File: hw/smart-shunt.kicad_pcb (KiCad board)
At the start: 2 copper layers, 80.3 x 50.3 mm, 36 parts, among them J1 V supply, J2 V bus <80, J3 V bus >80, J4 Conn_01x01_Female, J5 Conn_01x01_Female, J6 GND, U1 XL7005A, U2 INA228, U3 ESP-12F

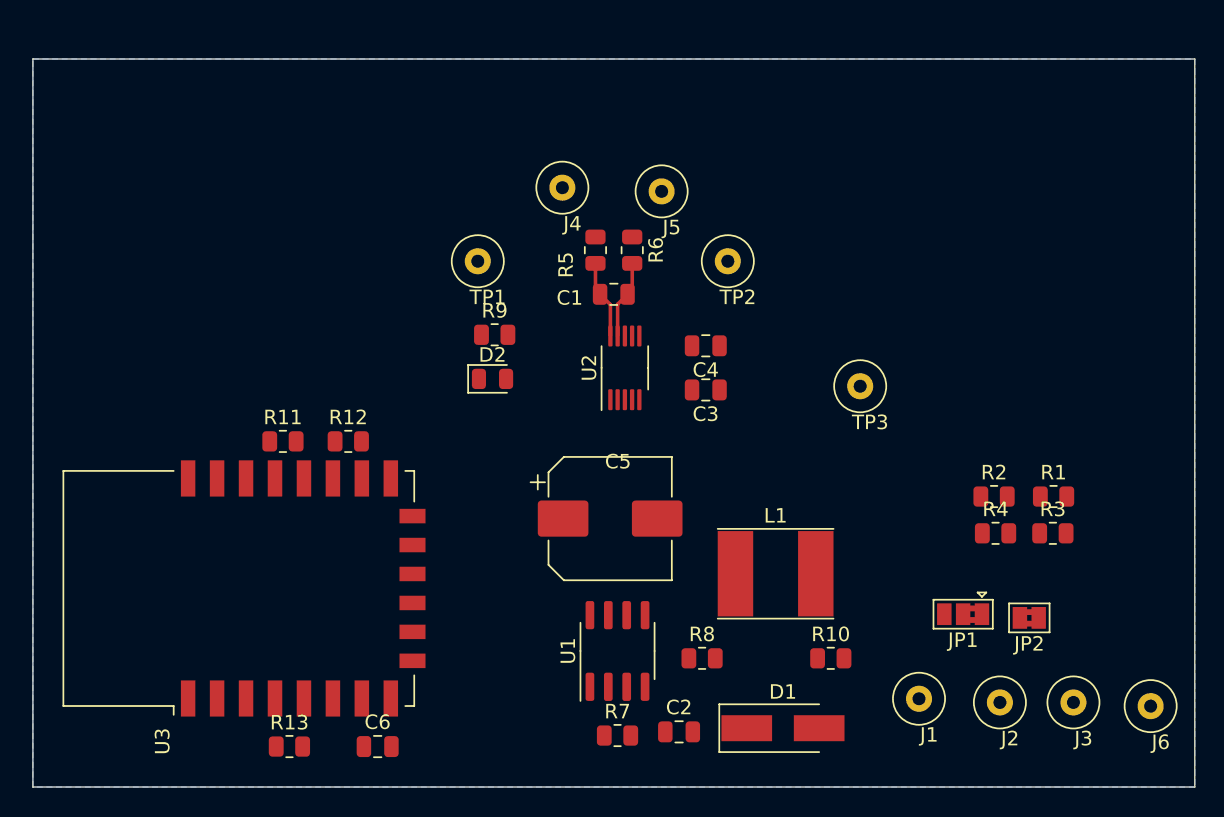
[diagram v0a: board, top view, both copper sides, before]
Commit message: finished pcb
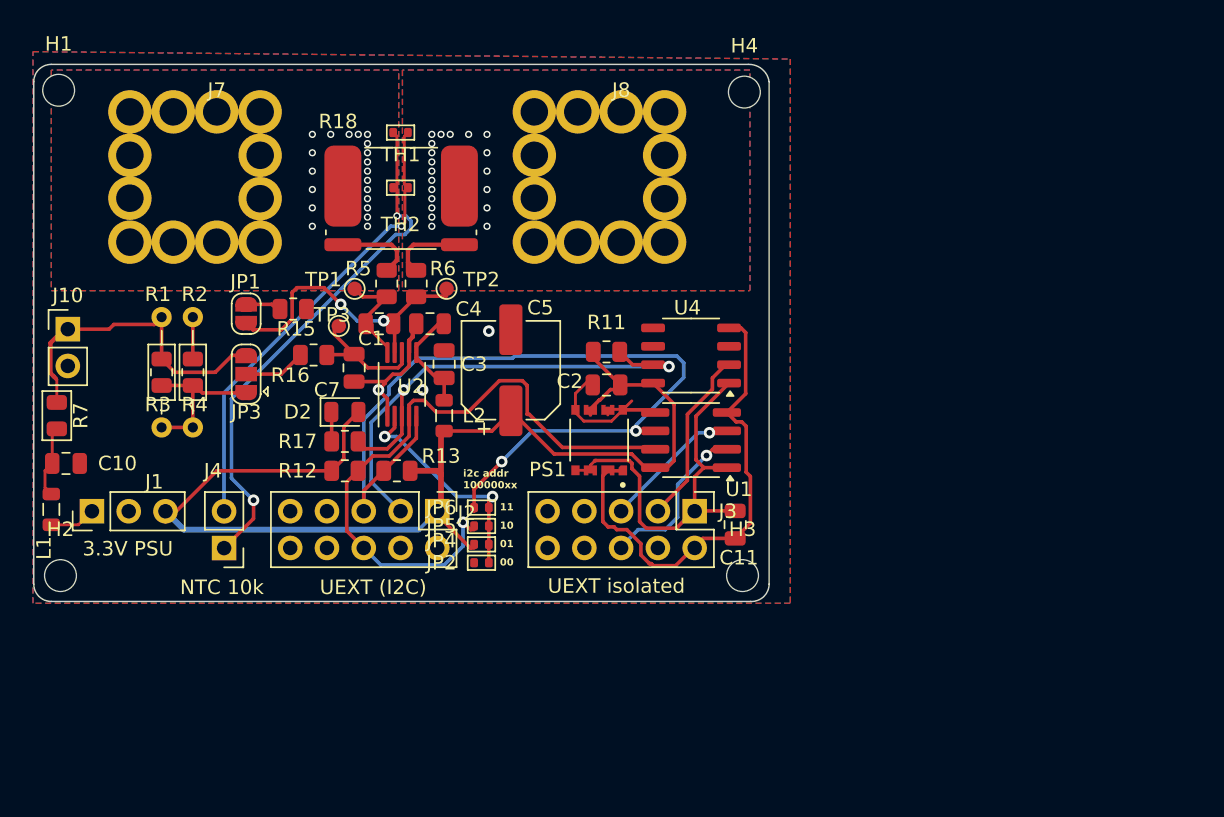
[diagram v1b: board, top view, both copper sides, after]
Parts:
- removed C6: 0.1uF, Capacitor_SMD:C_0805_2012Metric
- removed D1: SS310, Diode_SMD:D_SMA_Handsoldering
- removed J5: Conn_01x01_Female, TestPoint:TestPoint_Loop_D3.50mm_Drill0.9mm_Beaded
- removed J6: GND, TestPoint:TestPoint_Loop_D3.50mm_Drill0.9mm_Beaded
- removed R10: 33k, Resistor_SMD:R_0805_2012Metric
- removed R8, R9: 10k, Resistor_SMD:R_0805_2012Metric
- removed U3: ESP-12F, RF_Module:ESP-12E
- added C10: 1uF 100V, Capacitor_SMD:C_0805_2012Metric, F.Cu at (81.0, 99.6)
- added C11: 100nF, Capacitor_SMD:C_0805_2012Metric, F.Cu at (127.3, 103.8)
- added C7: 0.1uF, Capacitor_SMD:C_0805_2012Metric, F.Cu at (100.9, 93.0)
- added H1: MountingHole, MountingHole:MountingHole_2.2mm_M2, F.Cu at (80.5, 73.8)
- added H2: MountingHole, MountingHole:MountingHole_2.2mm_M2, F.Cu at (80.6, 107.3)
- added H3: MountingHole, MountingHole:MountingHole_2.2mm_M2, F.Cu at (127.8, 107.3)
- added H4: MountingHole, MountingHole:MountingHole_2.2mm_M2, F.Cu at (127.9, 73.9)
- added J10: Conn_01x02_Pin, Connector_PinHeader_2.54mm:PinHeader_1x02_P2.54mm_Vertical, F.Cu at (81.2, 90.3)
- added J7: Screw_Terminal_01x01, open-pe:Wuerth_PowerPlus_M5_Nut, F.Cu at (91.4, 81.3)
- added J8: Screw_Terminal_01x01, open-pe:Wuerth_PowerPlus_M5_Nut, F.Cu at (119.4, 81.3)
- added JP3: Jumper_3_Open, Jumper:SolderJumper-3_P1.3mm_Open_RoundedPad1.0x1.5mm, F.Cu at (93.5, 93.4)
- added JP4: SolderJumper_2_Open, PCM_Resistor_SMD_AKL:R_0402_1005Metric, F.Cu at (109.7, 105.2)
- added JP5: SolderJumper_2_Open, PCM_Resistor_SMD_AKL:R_0402_1005Metric, F.Cu at (109.7, 103.9)
- added JP6: SolderJumper_2_Open, PCM_Resistor_SMD_AKL:R_0402_1005Metric, F.Cu at (109.7, 102.6)
- added L2: LBR2012T101K, Inductor_SMD:L_0805_2012Metric, F.Cu at (107.1, 96.3)
- added PS1: MIE1W0505BGLVH-3R-Z, open-pe:CONV_MIE1W0505BGLVH-3R-Z, F.Cu at (117.9, 98.0)
- added R15: 10, Resistor_SMD:R_0805_2012Metric, F.Cu at (96.7, 88.9)
- added R16: 100, Resistor_SMD:R_0805_2012Metric, F.Cu at (98.1, 92.1)
- added R17: 10k, Resistor_SMD:R_0805_2012Metric, F.Cu at (100.3, 98.0)
- added R18: R_Shunt, Resistor_SMD:R_Shunt_Isabellenhuette_BVR4026, F.Cu at (104.2, 81.3)
- added TH1: Thermistor_NTC, PCM_Resistor_SMD_AKL:R_0402_1005Metric, F.Cu at (104.1, 76.7)
- added TH2: Thermistor_NTC, PCM_Resistor_SMD_AKL:R_0402_1005Metric, F.Cu at (104.1, 80.5)
- added U4: TPT7721-SO1R, Package_SO:SOP-8_3.9x4.9mm_P1.27mm, F.Cu at (124.2, 92.1)
- C2: value 33nF -> 100nF
- C5: value 100uF -> 22uF; footprint Capacitor_SMD:CP_Elec_8x10 -> Capacitor_SMD:CP_Elec_6.3x5.9
- J1: value V supply -> Conn_01x03_Socket; footprint TestPoint:TestPoint_Loop_D3.50mm_Drill0.9mm_Beaded -> Connector_PinHeader_2.54mm:PinHeader_1x03_P2.54mm_Vertical
- J2: value V bus <80 -> UEXT_Slave; footprint TestPoint:TestPoint_Loop_D3.50mm_Drill0.9mm_Beaded -> Connector_PinHeader_2.54mm:PinHeader_2x05_P2.54mm_Vertical
- J3: value V bus >80 -> UEXT_Slave2; footprint TestPoint:TestPoint_Loop_D3.50mm_Drill0.9mm_Beaded -> Connector_PinHeader_2.54mm:PinHeader_2x05_P2.54mm_Vertical
- J4: value Conn_01x01_Female -> Conn_01x02_Pin; footprint TestPoint:TestPoint_Loop_D3.50mm_Drill0.9mm_Beaded -> Connector_PinHeader_2.54mm:PinHeader_1x02_P2.54mm_Vertical
- JP1: value Jumper_3_Bridged12 -> Jumper_2_Open; footprint Jumper:SolderJumper-3_P1.3mm_Bridged2Bar12_Pad1.0x1.5mm -> Jumper:SolderJumper-2_P1.3mm_Open_RoundedPad1.0x1.5mm
- JP2: value Jumper_2_Open -> SolderJumper_2_Open; footprint Jumper:SolderJumper-2_P1.3mm_Bridged2Bar_Pad1.0x1.5mm -> PCM_Resistor_SMD_AKL:R_0402_1005Metric
- L1: value 100uH -> 22uH; footprint Inductor_SMD:L_Taiyo-Yuden_NR-60xx_HandSoldering -> Inductor_SMD:L_0805_2012Metric
- R1, R2: footprint Resistor_SMD:R_0805_2012Metric -> Resistor_THT:R_Axial_DIN0204_L3.6mm_D1.6mm_P7.62mm_Horizontal
- R7: value 33k -> 10; footprint Resistor_SMD:R_0805_2012Metric -> PCM_Resistor_SMD_AKL:R_0805_2012Metric
- TP1, TP2, TP3: footprint TestPoint:TestPoint_Loop_D3.50mm_Drill0.9mm_Beaded -> TestPoint:TestPoint_Pad_D1.0mm
- U1: value XL7005A -> TPT72616-SO1R
- moved R3 62.6 mm to (87.6, 93.3), turned to 90 degrees
- moved R1 61.8 mm to (87.6, 97.1), turned to 90 degrees
- moved J1 58.6 mm to (82.8, 102.9), turned to 90 degrees
- moved R2 56.7 mm to (89.8, 89.5), turned to -90 degrees
- moved R4 56.6 mm to (89.8, 93.3), turned to -90 degrees
- moved JP1 53.7 mm to (93.5, 89.2), turned to -90 degrees
- moved L1 50.2 mm to (80.0, 102.7), turned to 90 degrees
- moved R7 44.6 mm to (80.4, 96.3), turned to 90 degrees
- moved J2 41.1 mm to (106.7, 102.9), turned to -90 degrees
- moved JP2 38.0 mm to (109.7, 106.4)
- moved TP3 36.3 mm to (99.9, 90.1)
- moved J4 34.1 mm to (91.9, 105.4), turned to 180 degrees
- moved J3 29.3 mm to (124.5, 102.9), turned to -90 degrees
- moved C2 24.5 mm to (118.4, 94.1), turned to 180 degrees
- moved R11 23.2 mm to (118.4, 91.9), turned to 180 degrees
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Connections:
- C1 pad 2: Net-(TP2-Pad1) -> Net-(JP1-B)
- C2 pad 2: Net-(C2-Pad2) -> GND
- C3 pad 1: +3.3V -> Net-(U2-VS)
- C4 pad 1: +3.3V -> Net-(U2-VS)
- C5 pad 2: Net-(C5-Pad2) -> GND
- D2 pad 2: Alert -> +3.3V
- J1 pad 1: Net-(U1-Pad1) -> Net-(J1-Pin_1)
- J2 pad 1: Vbus -> +3.3V
- J3 pad 1: Net-(J3-Pad1) -> +3.3V2
- J4 pad 1: Net-(J4-Pad1) -> Net-(J4-Pin_1)
- JP1 pad 1: Vbus -> Net-(JP1-A)
- JP1 pad 2: Net-(JP1-Pad2) -> Net-(JP1-B)
- JP2 pad 1: Net-(JP2-Pad1) -> A0
- JP2 pad 2: Vbus -> GND
- L1 pad 1: Net-(D1-Pad1) -> Net-(J1-Pin_1)
- L1 pad 2: +3.3V -> Net-(C10-Pad2)
- R1 pad 1: Net-(JP2-Pad1) -> Net-(JP3-A)
- R1 pad 2: Net-(J3-Pad1) -> Vin
- R2 pad 2: Net-(JP2-Pad1) -> Net-(JP3-A)
- R3 pad 1: Net-(JP2-Pad1) -> Net-(JP3-A)
- R3 pad 2: Net-(J3-Pad1) -> Vin
- R4 pad 2: Net-(JP2-Pad1) -> Net-(JP3-A)
- R5 pad 1: Net-(J4-Pad1) -> Shunt+
- R6 pad 1: Net-(J5-Pad1) -> Shunt-
- R6 pad 2: Net-(TP2-Pad1) -> Net-(JP1-B)
- R7 pad 1: +3.3V -> Net-(C10-Pad2)
- R7 pad 2: Net-(C2-Pad2) -> Vin
- TP2 pad 1: Net-(TP2-Pad1) -> Net-(JP1-B)
- TP3 pad 1: Vbus -> Net-(U2-Vbus)
- U1 pad 1: Net-(U1-Pad1) -> +3.3V2
- U1 pad 2: Net-(D1-Pad1) -> SDA2
- U1 pad 3: Net-(C2-Pad2) -> SCL2
- U1 pad 4: Net-(C5-Pad2) -> GND2
- U1 pad 5: Net-(C5-Pad2) -> GND
- U1 pad 6: Net-(C5-Pad2) -> SCL
- U1 pad 7: Net-(C5-Pad2) -> SDA
- U1 pad 8: Net-(C5-Pad2) -> +3.3V
- U2 pad 2: GND -> A0
- U2 pad 6: +3.3V -> Net-(U2-VS)
- U2 pad 8: Vbus -> Net-(U2-Vbus)
- U2 pad 9: Net-(TP2-Pad1) -> Net-(JP1-B)
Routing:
- net +3.3V: track 0.00 -> 81.9 mm
- net SCL: track 0.00 -> 60.2 mm, vias 0 -> 2
- net SDA: track 0.00 -> 44.8 mm, vias 0 -> 1
- net Alert: track 0.00 -> 39.3 mm, vias 0 -> 2
- net Net-(J4-Pin_1): track 0.00 -> 36.6 mm, vias 0 -> 2
- net GND2: track 0.00 -> 33.9 mm
- net Net-(J4-Pin_2): track 0.00 -> 32.2 mm, vias 0 -> 1
- net +3.3V2: track 0.00 -> 28.2 mm
- net GND: track 0.00 -> 23.2 mm, vias 0 -> 3
- net Vin: track 0.00 -> 21.7 mm
- net Net-(JP1-B): track 0.00 -> 20.7 mm, vias 0 -> 2
- net A0: track 0.00 -> 14.9 mm, vias 0 -> 2
- net Alert2: track 0.00 -> 12.2 mm
- net SDA2: track 0.00 -> 11.4 mm, vias 0 -> 1
- net Net-(JP3-A): track 0.00 -> 10.6 mm
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- added copper zone on F.Cu, net GND
- added copper zone on B.Cu, net P+
- added copper zone on F.Cu, net P+
- added copper zone on B.Cu, net P-
- added copper zone on F.Cu, net P-
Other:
- board size 80.3 x 50.3 mm -> 50.8 x 37.1 mm
- board text added: "00"
- board text added: "01"
- board text added: "10"
- board text added: "11"
- board text added: "3.3V PSU"
- board text added: "NTC 10k"
- board text added: "UEXT (I2C)"
- board text added: "UEXT isolated"
- board text added: "i2c addr 100000xx"
- board text removed: "use double footprints for resistors (THT and SMD) add filter connectors"
